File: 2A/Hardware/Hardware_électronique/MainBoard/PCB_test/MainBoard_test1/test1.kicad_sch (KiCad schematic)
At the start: 28 parts, among them J3 Conn_02x10_Odd_Even, Q1 PMOS, U3 AP64500Q

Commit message: last minute update
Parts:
- BT1: footprint Connector_AMASS:AMASS_XT60PW-F_1x02_P7.20mm_Horizontal -> Connector_AMASS:AMASS_XT60-F_1x02_P7.20mm_Vertical
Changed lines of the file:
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@@
 			)
 		)
-		(property "Footprint" "Connector_AMASS:AMASS_XT60PW-F_1x02_P7.20mm_Horizontal"
+		(property "Footprint" "Connector_AMASS:AMASS_XT60-F_1x02_P7.20mm_Vertical"
 			(at 36.83 149.606 90)
 			(effects

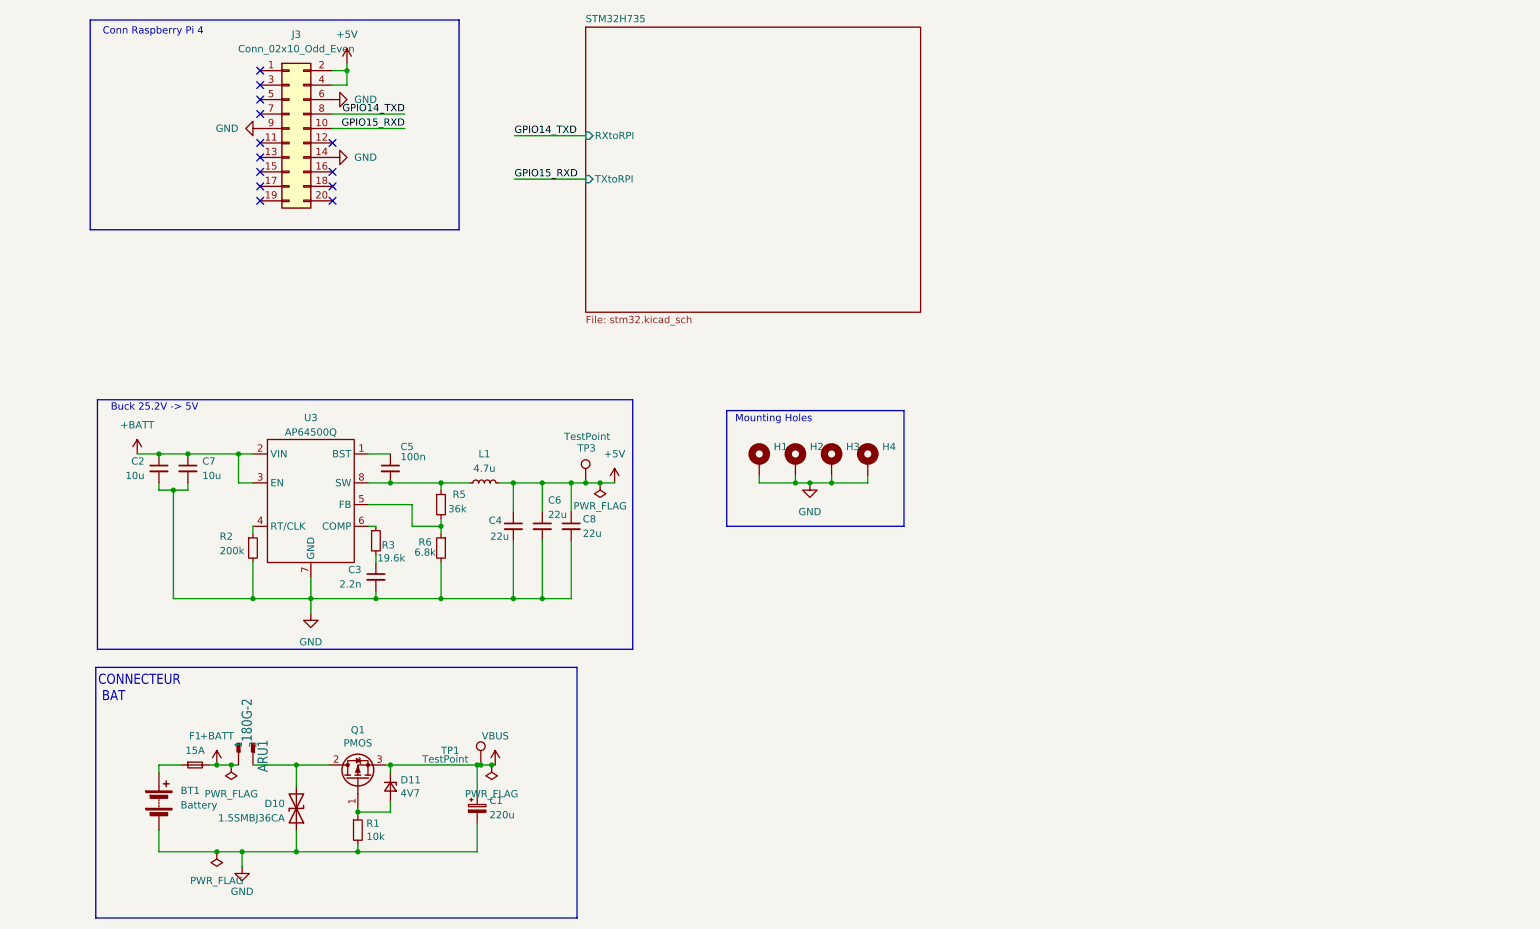
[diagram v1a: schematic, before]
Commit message: pcb edits
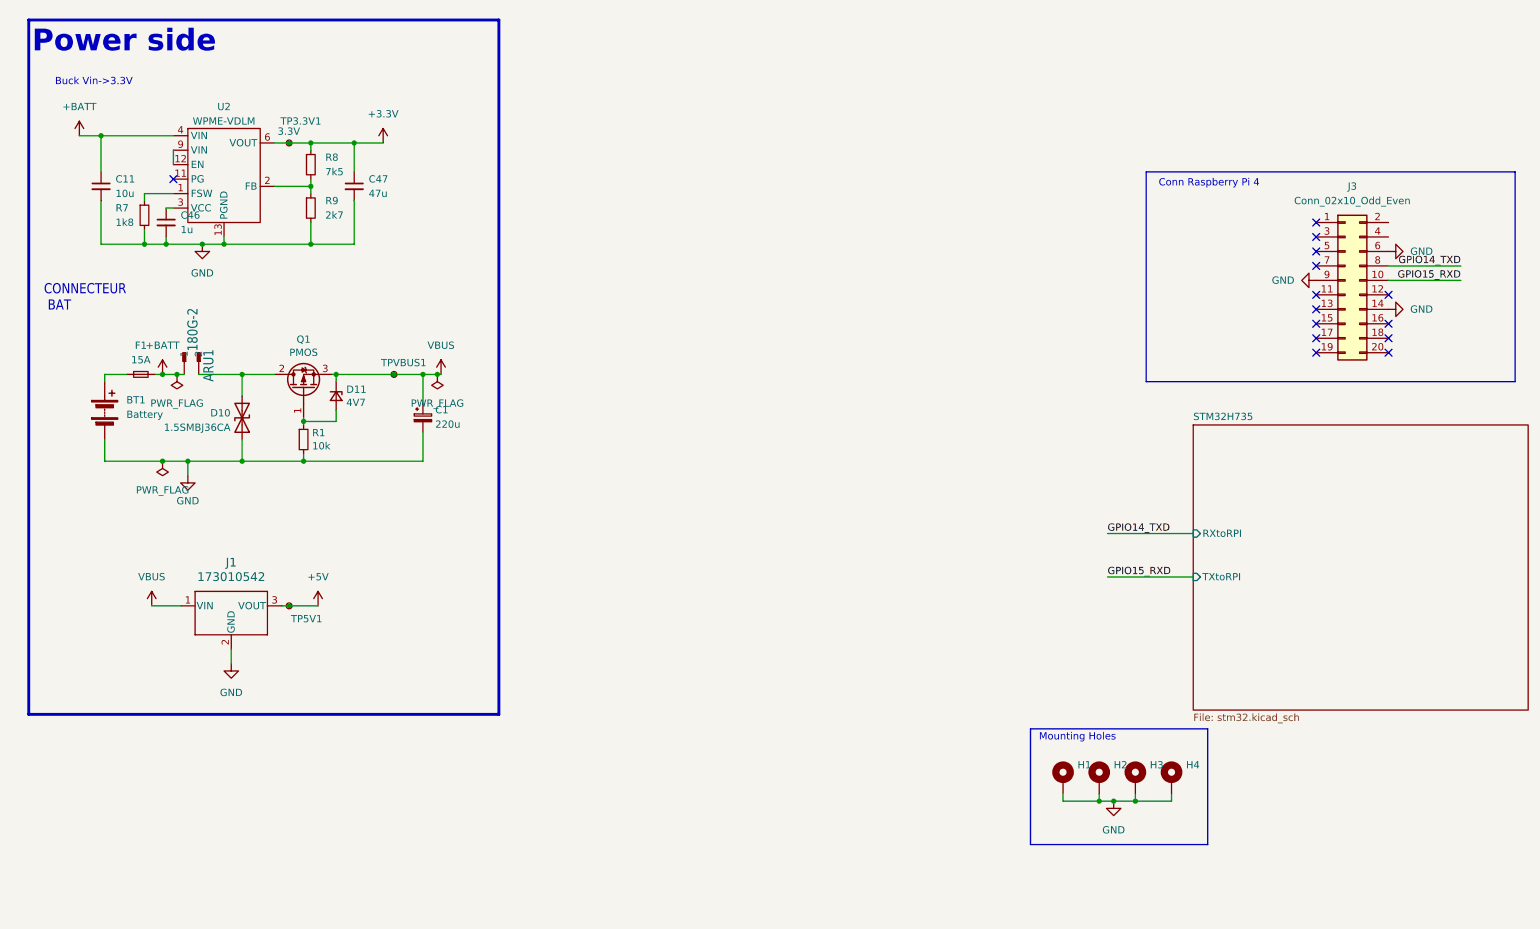
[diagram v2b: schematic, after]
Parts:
- removed C2, C7: 10u, Capacitor_SMD:C_0805_2012Metric, symbol Device:C_Small
- removed C3: 2.2n, Capacitor_SMD:C_0402_1005Metric, symbol Device:C_Small
- removed C4, C6, C8: 22u, Capacitor_SMD:C_0805_2012Metric, symbol Device:C_Small
- removed C5: 100n, Capacitor_SMD:C_0402_1005Metric, symbol Device:C_Small
- removed L1: 4.7u, MainBoard:PA5432.472NLT, symbol Device:L_Small
- removed R2: 200k, Resistor_SMD:R_0402_1005Metric, symbol Device:R_Small
- removed R3: 19.6k, Resistor_SMD:R_0402_1005Metric, symbol Device:R_Small
- removed R5: 36k, Resistor_SMD:R_0402_1005Metric, symbol Device:R_Small
- removed R6: 6.8k, Resistor_SMD:R_0402_1005Metric, symbol Device:R_Small
- removed TP1, TP3: TestPoint, TestPoint:TestPoint_Pad_D2.0mm, symbol Connector:TestPoint
- removed U3: AP64500Q, Package_SO:SOIC-8-1EP_3.9x4.9mm_P1.27mm_EP2.95x4.9mm_Mask2.71x3.4mm, symbol Custom:AP64500Q
- added C11: 10u, Capacitor_SMD:C_0805_2012Metric, symbol Device:C_Small
- added C46: 1u, Capacitor_SMD:C_0603_1608Metric, symbol Device:C_Small
- added C47: 47u, Capacitor_SMD:C_0805_2012Metric, symbol Device:C_Small
- added J1: 173010542, Connector_PinHeader_2.54mm:PinHeader_1x03_P2.54mm_Vertical, symbol 173010542_5V_Buck:173010542
- added R7: 1k8, Resistor_SMD:R_0402_1005Metric, symbol Device:R_Small
- added R8: 7k5, Resistor_SMD:R_0402_1005Metric, symbol Device:R_Small
- added R9: 2k7, Resistor_SMD:R_0402_1005Metric, symbol Device:R_Small
- added TP3.3V1, TP5V1, TPVBUS1: 3.3V, TestPoint:TestPoint_Pad_D1.0mm, symbol Connector:TestPoint_Small
- added U2: WPME-VDLM, CustomLibrary:WPME-VDLM, symbol Custom:Buck171013801
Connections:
- net +5V: now also J1.3 (VOUT), TP5V1.1; no longer J3.2 (Pin_2), J3.4 (Pin_4)
- net +BATT: now also C11.1, U2.4 (VIN), U2.5 (VIN)
- net GND: now also C11.2, C46.2, C47.2, J1.2 (GND), R7.2, R9.2, U2.10 (AGND), U2.13 (PGND)
- net VBUS: now also J1.1 (VIN), TPVBUS1.1
- new net: R8.2, R9.1, U2.2 (FB)
- new net: R7.1, U2.1 (FSW)
- new net: U2.12 (EN), U2.9 (VIN)
- new net: C46.1, U2.3 (VCC)
- new net +3.3V: C47.1, R8.1, TP3.3V1.1, U2.6 (VOUT), U2.7 (VOUT)
- no-connect marks 13 -> 14
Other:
- note added: "Buck Vin->3.3V"
- note added: "Power side"
- note removed: "Buck 25.2V -> 5V"
- moved on the sheet: ARU1, BT1, C1, D10, D11, F1, H1, H2, H3, H4, J3, Q1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
